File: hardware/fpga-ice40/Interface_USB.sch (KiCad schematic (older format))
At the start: 12 parts, among them J5 USB_B_Micro, U9 FT245RL

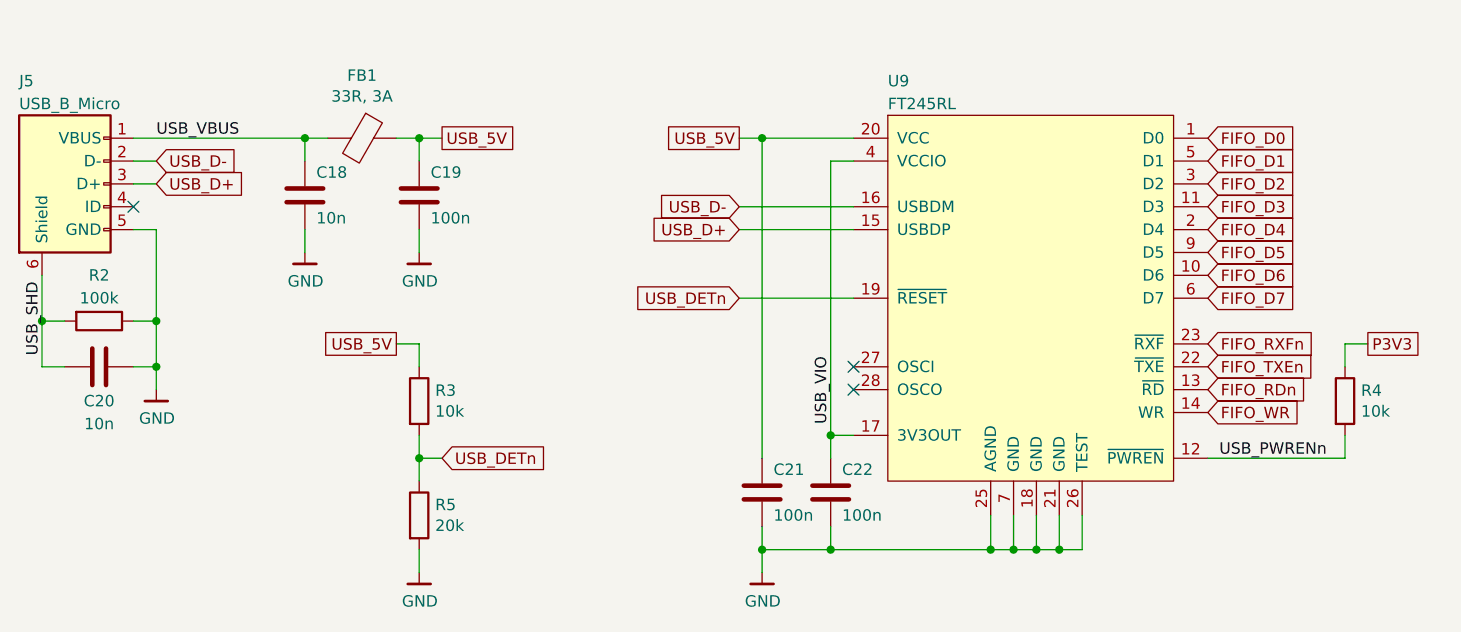
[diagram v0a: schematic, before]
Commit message: Completed schematic review
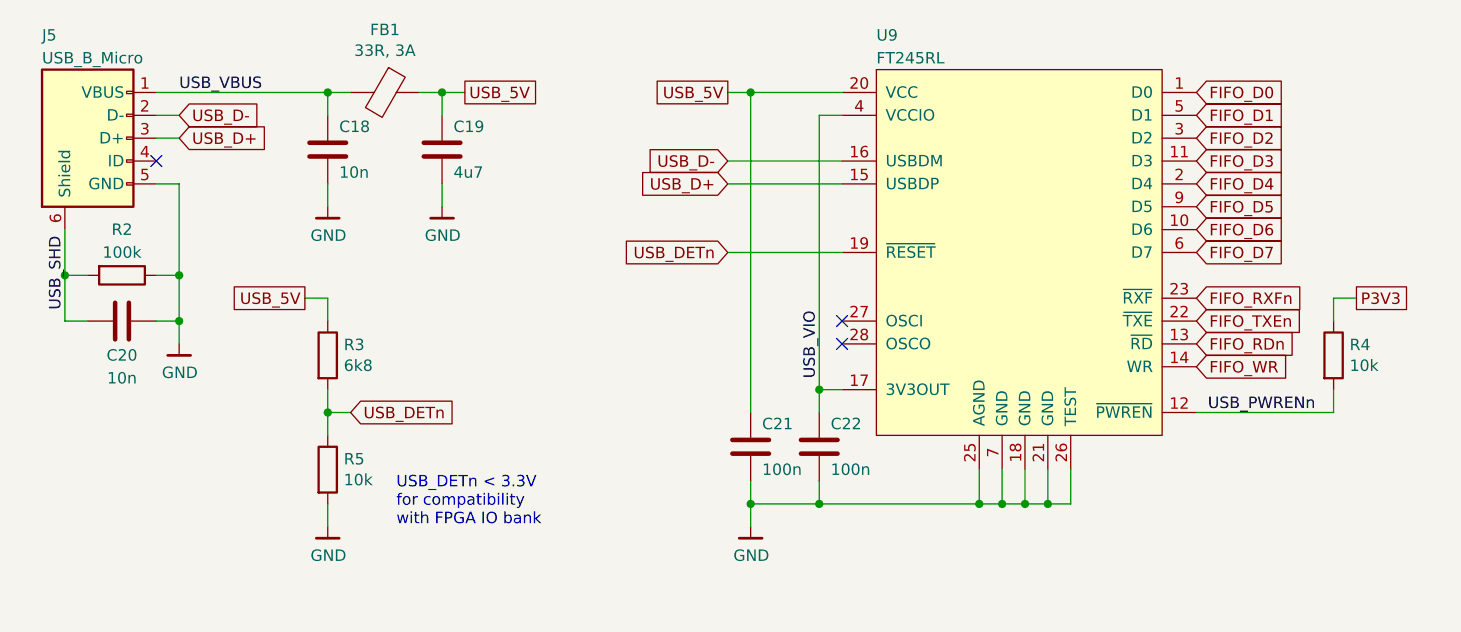
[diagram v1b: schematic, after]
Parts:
- C19: value 100n -> 4u7; MPN CL10B104KB8NNNC -> CL10A475KA8NQNC
- R3: value 10k -> 6k8; MPN RC0603FR-0710KL -> RC0603FR-076K8L
- R5: value 20k -> 10k; MPN RC0603JR-0720KL -> RC0603FR-0710KL
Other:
- note added: "USB_DETn < 3.3V\nfor compatibility\nwith FPGA IO bank"
- moved on the sheet: C18, C19, C20, C21, C22, FB1, J5, R2, R3, R4, R5, U9
